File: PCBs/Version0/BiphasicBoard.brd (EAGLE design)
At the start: 25.9 x 16.5 mm, 11 parts

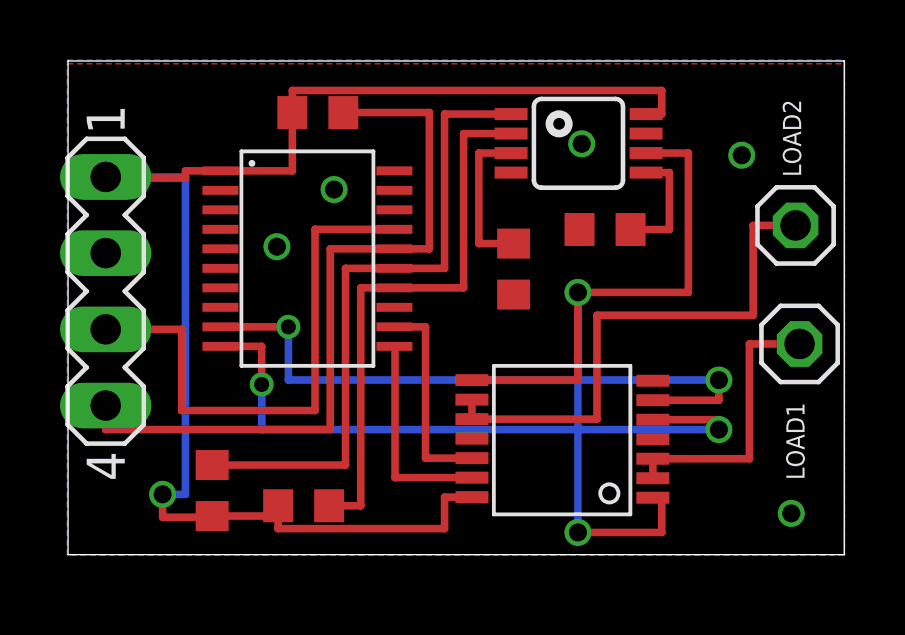
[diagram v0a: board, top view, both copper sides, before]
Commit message: Updated Library Parts
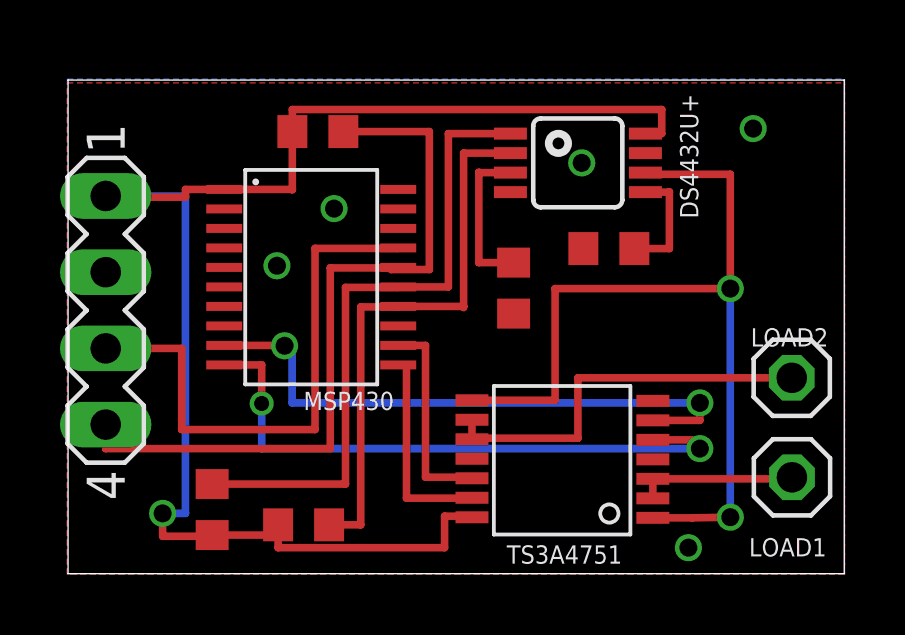
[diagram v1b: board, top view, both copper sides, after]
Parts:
- removed DS4432: (no value), DS4432U+:DS4432U+
- removed R1, R2: (no value), resistor:R0603
- removed U$1: G2X[1/5]2---PW20, TI_MSP430_v16:PW20
- added DS4432U+: (no value), BiphasicBoard:8_PIN
- added MSP430: (no value), BiphasicBoard:20_PIN
- added R_INPUT_FS0, R_INPUT_FS1: (no value), BiphasicBoard:R0603
- LOAD1, LOAD2: device pinhead:1X01 -> BiphasicBoard:1X01
- R_PULLUP_RST, R_PULLUP_SCL, R_PULLUP_SDA: device resistor:R0603 -> BiphasicBoard:R0603
- SV1: device con-lstb:MA04-1 -> BiphasicBoard:MA04-1
- TS3A4751: device TS3A4751:TS3A4751#2 -> BiphasicBoard:14_PIN
- moved LOAD2 5.08 mm to (24.1, 6.55)
- moved LOAD1 4.45 mm to (24.2, 3.23)
- moved TS3A4751 2.32 mm to (16.3, 3.05), turned to 180 degrees
- moved R_PULLUP_SDA 0.64 mm to (4.83, 2.16)
- moved R_PULLUP_SCL 0.64 mm to (7.87, 1.65)
- moved R_PULLUP_RST 0.63 mm to (8.35, 14.8)
- moved SV1 0.63 mm to (1.28, 8.80)
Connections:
- removed net N$10: TS3A4751.13, U$1.11
- removed net N$11: TS3A4751.12, U$1.12
- new net IN1: MSP430.11, TS3A4751.13
- new net IN4: MSP430.12, TS3A4751.12
- net CURRENT0: now also DS4432U+.6; no longer DS4432.6
- net GND: now also DS4432U+.4, MSP430.20, R_INPUT_FS0.1, R_INPUT_FS1.1; no longer DS4432.4, R1.1, R2.1, U$1.20
- net N$1: now also DS4432U+.2, MSP430.14; no longer DS4432.2, U$1.14
- net N$2: now also DS4432U+.1, MSP430.15; no longer DS4432.1, U$1.15
- net N$4: now also MSP430.10; no longer U$1.10
- net N$8: now also DS4432U+.5, R_INPUT_FS0.2; no longer DS4432.5, R2.2
- net N$9: now also MSP430.9; no longer U$1.9
- net TEST: now also MSP430.17; no longer U$1.17
- net VDD: now also DS4432U+.8, MSP430.1; no longer DS4432.8, U$1.1
- net VIA1: now also DS4432U+.3, R_INPUT_FS1.2; no longer DS4432.3, R1.2
- net _RST: now also MSP430.16; no longer U$1.16
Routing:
- net N$10: track 7.07 -> 0.00 mm
- net N$11: track 6.96 -> 0.00 mm
- net IN1: track 0.00 -> 6.91 mm
- net IN4: track 0.00 -> 6.89 mm
- net LOAD2: track 17.9 -> 13.3 mm
- net LOAD1: track 9.37 -> 5.34 mm
- net N$4: track 21.9 -> 20.5 mm
- net N$9: track 21.3 -> 19.9 mm
- net CURRENT0: track 28.4 -> 29.2 mm
- net _RST: track 25.0 -> 25.6 mm
